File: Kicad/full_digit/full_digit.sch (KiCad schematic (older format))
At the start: 49 parts, among them J1 CONN_8, J10 CONN_01X03, J11 CONN_01X12, J12 CONN_01X12, J13 CONN_01X08, J14 CONN_01X06, J15 CONN_01X10, J16 CONN_01X08, J17 CONN_01X17, J18 CONN_01X17, J19 RASM722X, J2 CONN_8, J3 CONN_8, J4 CONN_8, J5 CONN_8, J6 CONN_8, J7 CONN_8, J8 CONN_8, J9 CONN_01X03, U1 TLC5917, X1 MTHOLE, X2 MTHOLE, X3 MTHOLE, X4 MTHOLE

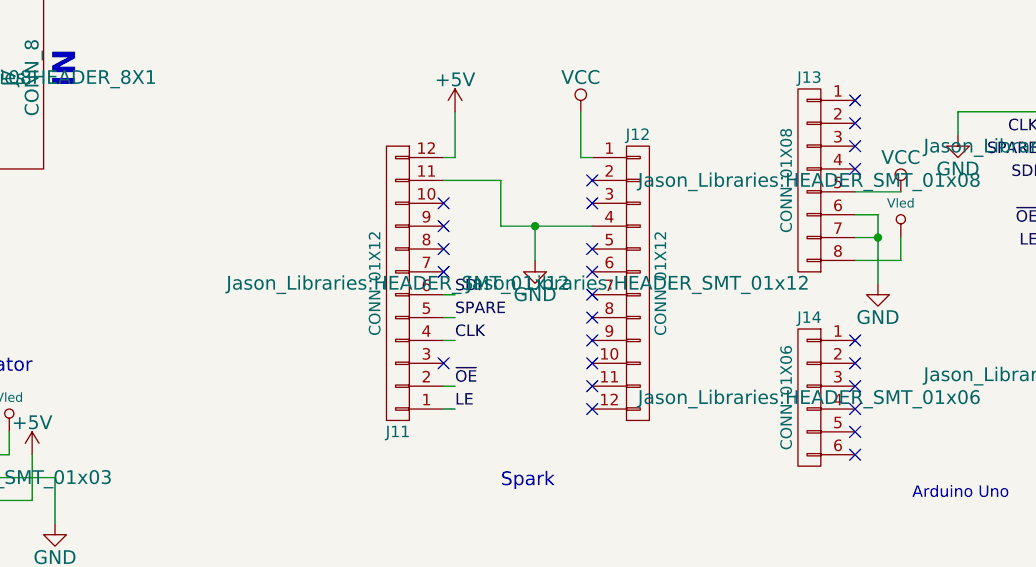
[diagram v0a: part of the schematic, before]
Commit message: Rev 3 Final Draft
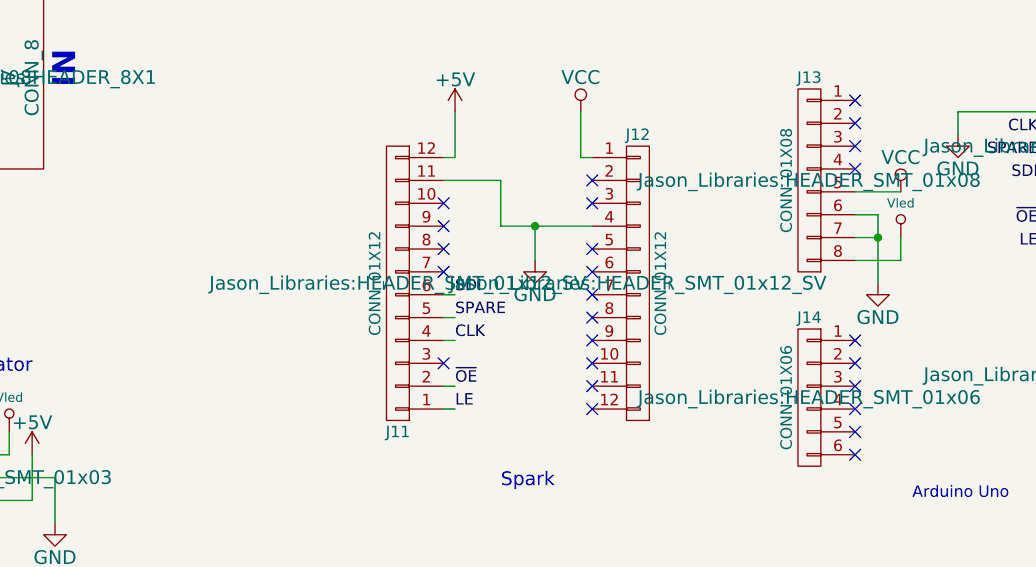
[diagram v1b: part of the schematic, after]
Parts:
- J11, J12: footprint Jason_Libraries:HEADER_SMT_01x12 -> Jason_Libraries:HEADER_SMT_01x12_SV
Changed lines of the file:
@@
 F 0 "J12" H 6650 6350 50  0000 C CNN
 F 1 "CONN_01X12" V 6750 5700 50  0000 C CNN
-F 2 "Jason_Libraries:HEADER_SMT_01x12" H 6650 5700 60  0000 C CNN
+F 2 "Jason_Libraries:HEADER_SMT_01x12_SV" H 6650 5700 60  0000 C CNN
 F 3 "" H 6650 5700 60  0000 C CNN
 	1    6650 5700
@@
 F 0 "J11" H 5600 6350 50  0000 C CNN
 F 1 "CONN_01X12" V 5700 5700 50  0000 C CNN
-F 2 "Jason_Libraries:HEADER_SMT_01x12" H 5600 5700 60  0000 C CNN
+F 2 "Jason_Libraries:HEADER_SMT_01x12_SV" H 5600 5700 60  0000 C CNN
 F 3 "" H 5600 5700 60  0000 C CNN
 	1    5600 5700
